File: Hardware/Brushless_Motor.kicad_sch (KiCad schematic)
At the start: 1 part, among them J8 Turbo_Fan

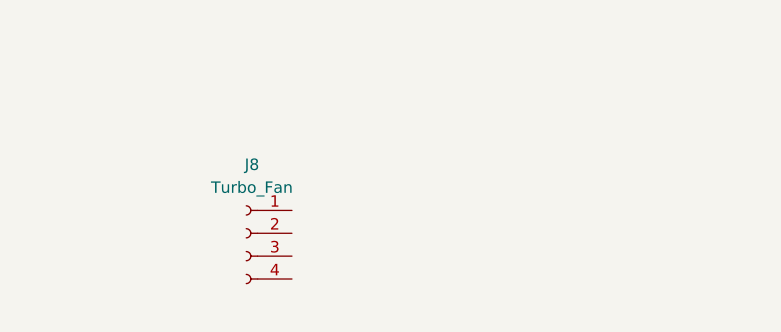
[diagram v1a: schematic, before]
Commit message: Update PCB
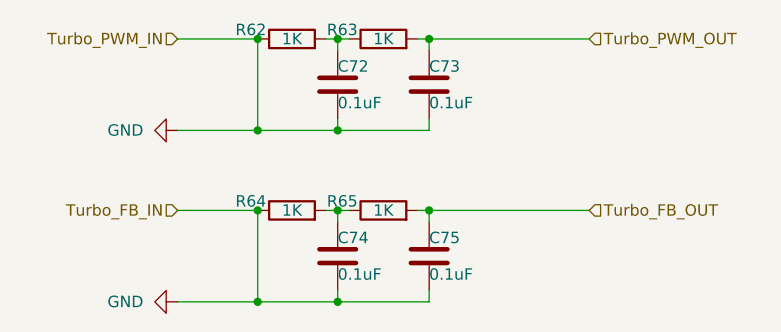
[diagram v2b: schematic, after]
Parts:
- removed J8: Turbo_Fan, symbol Connector:Conn_01x04_Socket
- added C72, C73, C74, C75: 0.1uF, Capacitor_SMD:C_0603_1608Metric, symbol Library:C
- added R62, R63, R64, R65: 1K, Resistor_SMD:R_0603_1608Metric, symbol Library:R
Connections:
- new net: C72.2, R62.2, R63.1
- new net: C74.2, R64.2, R65.1
- new net GND: C72.1, C73.1, C74.1, C75.1, R62.1, R64.1
- new net Turbo_FB_OUT: C75.2, R65.2
- new net Turbo_PWM_OUT: C73.2, R63.2
